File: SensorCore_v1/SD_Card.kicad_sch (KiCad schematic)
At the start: 4 parts, among them J1 Micro_SD_Card_Det1, U4 EMIF06-MSD02N16

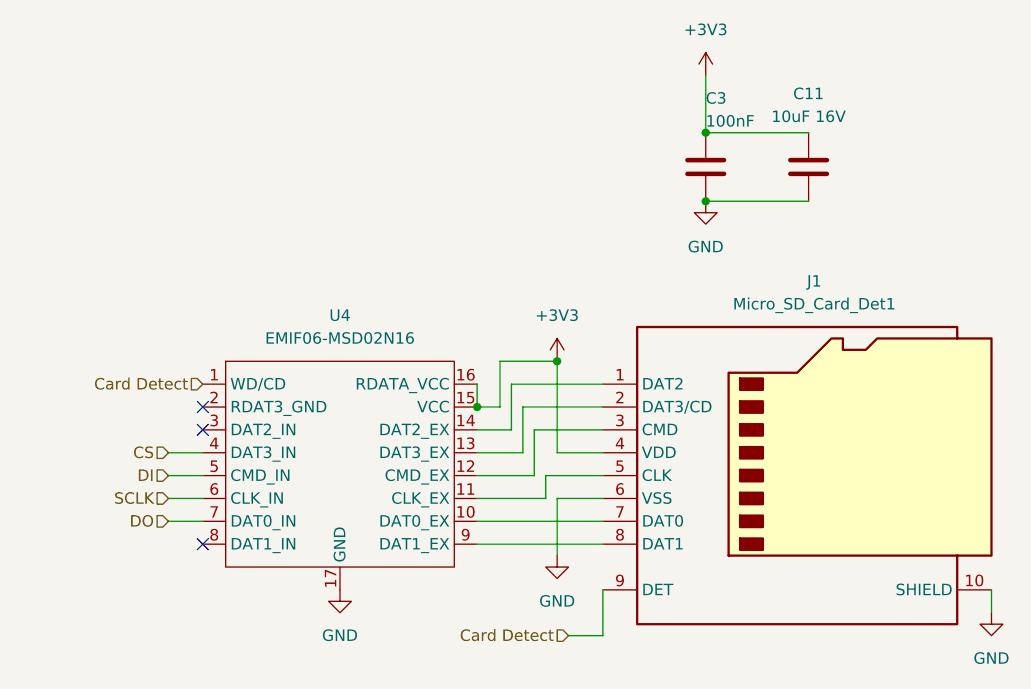
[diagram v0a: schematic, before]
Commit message: Preliminary design done
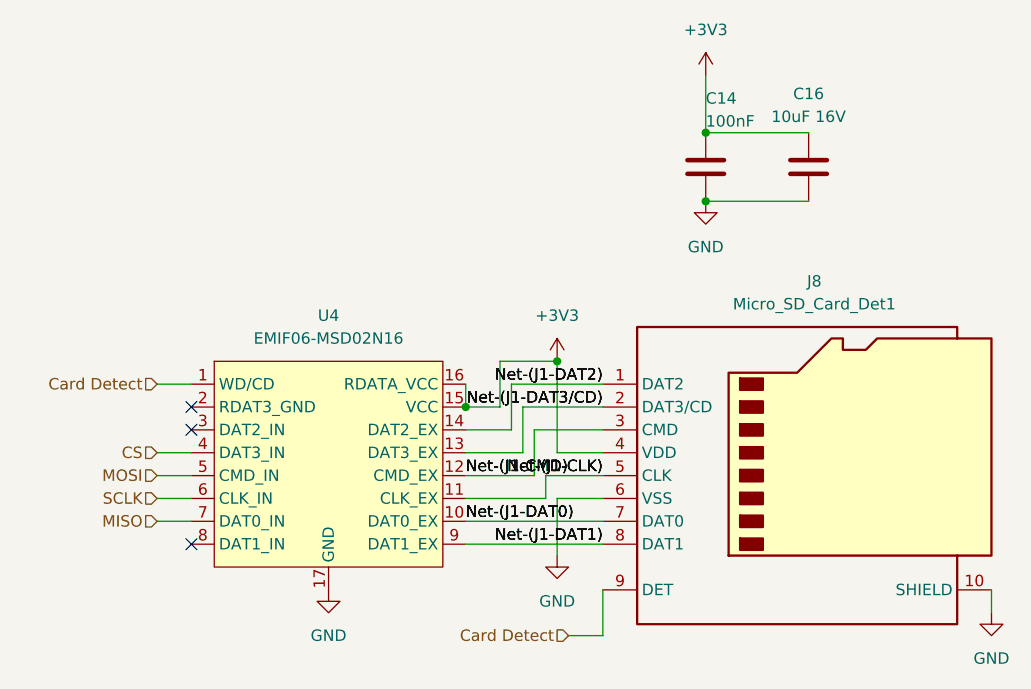
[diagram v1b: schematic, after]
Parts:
- C14: renamed from C3; footprint Resistor_SMD:R_0603_1608Metric_Pad0.98x0.95mm_HandSolder -> Capstone Footprints:C_0603_1608Metric_Pad1.08x0.95mm_HandSolder; symbol Device:C -> Project:C; KiLib_Generator (none) -> SMD_2terminal_chip_molded
- C16: renamed from C11; footprint Capacitor_SMD:C_0805_2012Metric_Pad1.18x1.45mm_HandSolder -> Capstone Footprints:C_0805_2012Metric_Pad1.18x1.45mm_HandSolder; symbol Device:C -> Project:C
- J8: renamed from J1; footprint Extra_Footprints:CUI_MSD-11-A -> Capstone Footprints:CUI_MSD-11-A; symbol Connector:Micro_SD_Card_Det1 -> Project:Micro_SD_Card_Det1
- U4: footprint Package_DFN_QFN:OnSemi_UDFN-16-1EP_1.35x3.3mm_P0.4mm_EP0.4x2.8mm -> Capstone Footprints:OnSemi_UDFN-16-1EP_1.35x3.3mm_P0.4mm_EP0.4x2.8mm; symbol Extra_Symbols:EMIF06-MSD02N16 -> Project:EMIF06-MSD02N16
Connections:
- net Net-(J1-DAT0): now reaches J8.7 (DAT0), U4.10 (DAT0_EX)
- net Net-(J1-CLK): now reaches J8.5 (CLK), U4.11 (CLK_EX)
- net Net-(J1-CMD): now reaches J8.3 (CMD), U4.12 (CMD_EX)
- net Net-(J1-DAT3/CD): now reaches J8.2 (DAT3/CD), U4.13 (DAT3_EX)
- net Net-(J1-DAT2): now reaches J8.1 (DAT2), U4.14 (DAT2_EX)
- net Net-(J1-DAT1): now reaches J8.8 (DAT1), U4.9 (DAT1_EX)
- net DI renamed MOSI
- net DO renamed MISO

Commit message: SensorCore v1.0 - Approved
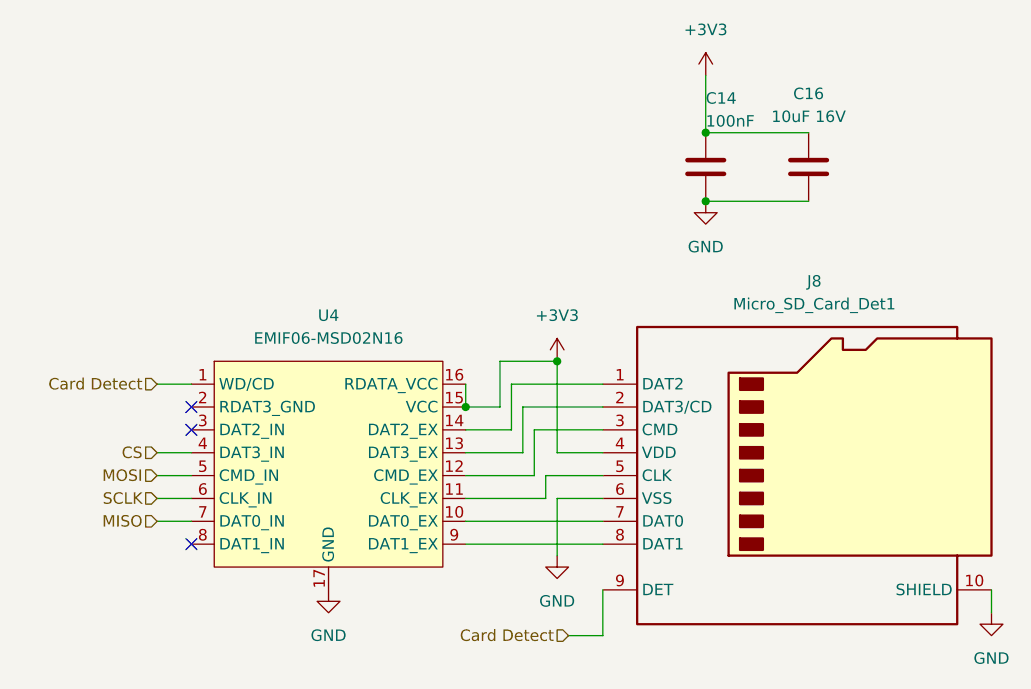
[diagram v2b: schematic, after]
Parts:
- U4: Digikey Part (none) -> EMIF06-MSD02N16
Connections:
- net Net-(J1-CLK): no longer names the net of J8.5 (CLK), U4.11 (CLK_EX)
- net Net-(J1-CMD): no longer names the net of J8.3 (CMD), U4.12 (CMD_EX)
- net Net-(J1-DAT0): no longer names the net of J8.7 (DAT0), U4.10 (DAT0_EX)
- net Net-(J1-DAT1): no longer names the net of J8.8 (DAT1), U4.9 (DAT1_EX)
- net Net-(J1-DAT2): no longer names the net of J8.1 (DAT2), U4.14 (DAT2_EX)
- net Net-(J1-DAT3/CD): no longer names the net of J8.2 (DAT3/CD), U4.13 (DAT3_EX)
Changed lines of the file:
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@@
 		(title "Sensor Core PCB")
 		(date "2026-09-08")
-		(rev "v1.1")
+		(rev "v1.0")
 		(company "Vector Drive (MXET)")
 		(comment 1 "Lucas Ngo")
@@
 			(width 0)
 			(type default)
-		)
-	)
-	(label "Net-(J1-DAT2)"
-		(at 140.97 86.36 180)
-		(effects
-			(font
-				(size 1.27 1.27)
-			)
-			(justify right bottom)
-		)
-	)
-	(label "Net-(J1-CLK)"
-		(at 140.97 96.52 180)
-		(effects
-			(font
-				(size 1.27 1.27)
-			)
-			(justify right bottom)
-		)
-	)
-	(label "Net-(J1-DAT3{slash}CD)"
-		(at 140.97 88.9 180)
-		(effects
-			(font
-				(size 1.27 1.27)
-			)
-			(justify right bottom)
-		)
-	)
-	(label "Net-(J1-CLK)"
-		(at 140.97 96.52 180)
-		(effects
-			(font
-				(size 1.27 1.27)
-			)
-			(justify right bottom)
-		)
-	)
-	(label "Net-(J1-DAT3{slash}CD)"
-		(at 140.97 88.9 180)
-		(effects
-			(font
-				(size 1.27 1.27)
-			)
-			(justify right bottom)
-		)
-	)
-	(label "Net-(J1-DAT1)"
-		(at 140.97 104.14 180)
-		(effects
-			(font
-				(size 1.27 1.27)
-			)
-			(justify right bottom)
-		)
-	)
-	(label "Net-(J1-CMD)"
-		(at 125.73 96.52 0)
-		(effects
-			(font
-				(size 1.27 1.27)
-			)
-			(justify left bottom)
-		)
-	)
-	(label "Net-(J1-DAT0)"
-		(at 125.73 101.6 0)
-		(effects
-			(font
-				(size 1.27 1.27)
-			)
-			(justify left bottom)
-		)
-	)
-	(label "Net-(J1-DAT0)"
-		(at 125.73 101.6 0)
-		(effects
-			(font
-				(size 1.27 1.27)
-			)
-			(justify left bottom)
-		)
-	)
-	(label "Net-(J1-DAT2)"
-		(at 140.97 86.36 180)
-		(effects
-			(font
-				(size 1.27 1.27)
-			)
-			(justify right bottom)
-		)
-	)
-	(label "Net-(J1-DAT1)"
-		(at 140.97 104.14 180)
-		(effects
-			(font
-				(size 1.27 1.27)
-			)
-			(justify right bottom)
-		)
-	)
-	(label "Net-(J1-CMD)"
-		(at 125.73 96.52 0)
-		(effects
-			(font
-				(size 1.27 1.27)
-			)
-			(justify left bottom)
 		)
 	)
@@
 			(at 110.49 95.25 0)
 			(hide yes)
+			(show_name no)
+			(do_not_autoplace no)
+			(effects
+				(font
+					(size 1.27 1.27)
+				)
+			)
+		)
+		(property "Digikey Part" "EMIF06-MSD02N16"
+			(at 110.49 95.25 0)
+			(hide yes)
